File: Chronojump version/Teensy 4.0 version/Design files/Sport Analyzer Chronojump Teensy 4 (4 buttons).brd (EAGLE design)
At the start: 122.7 x 68.6 mm, 40 parts, among them IC2 7805DT, Q1 MMBT4403, Q2 BSS138, Q3 BSS138, SW1 C&K_COMPONENTS_D6R40F1LFSC&K_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, SW2 C&K_COMPONENTS_D6R40F1LFSC&K_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, SW3 C&K_COMPONENTS_D6R40F1LFSC&K_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, SW4 C&K_COMPONENTS_D6R40F1LFSC&K_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, U1 HX711

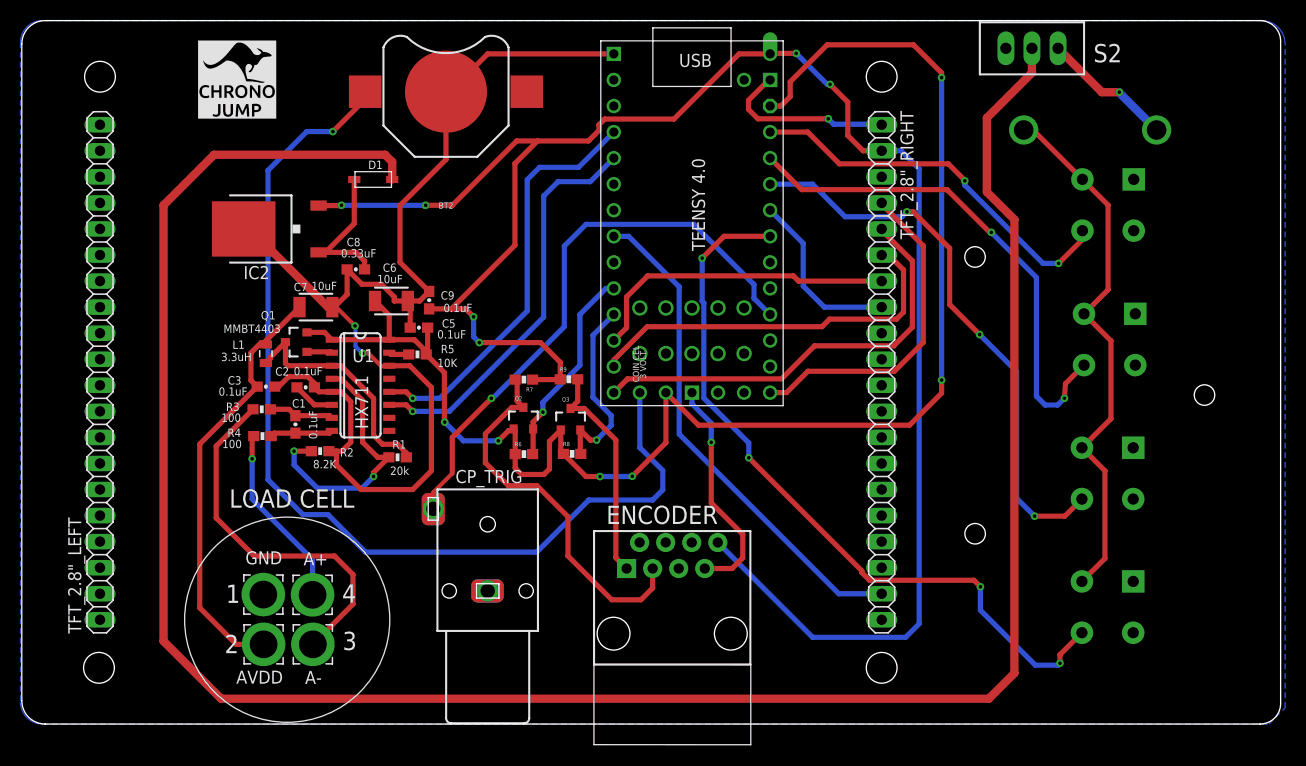
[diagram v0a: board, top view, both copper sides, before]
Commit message: RTC DS1302 v1
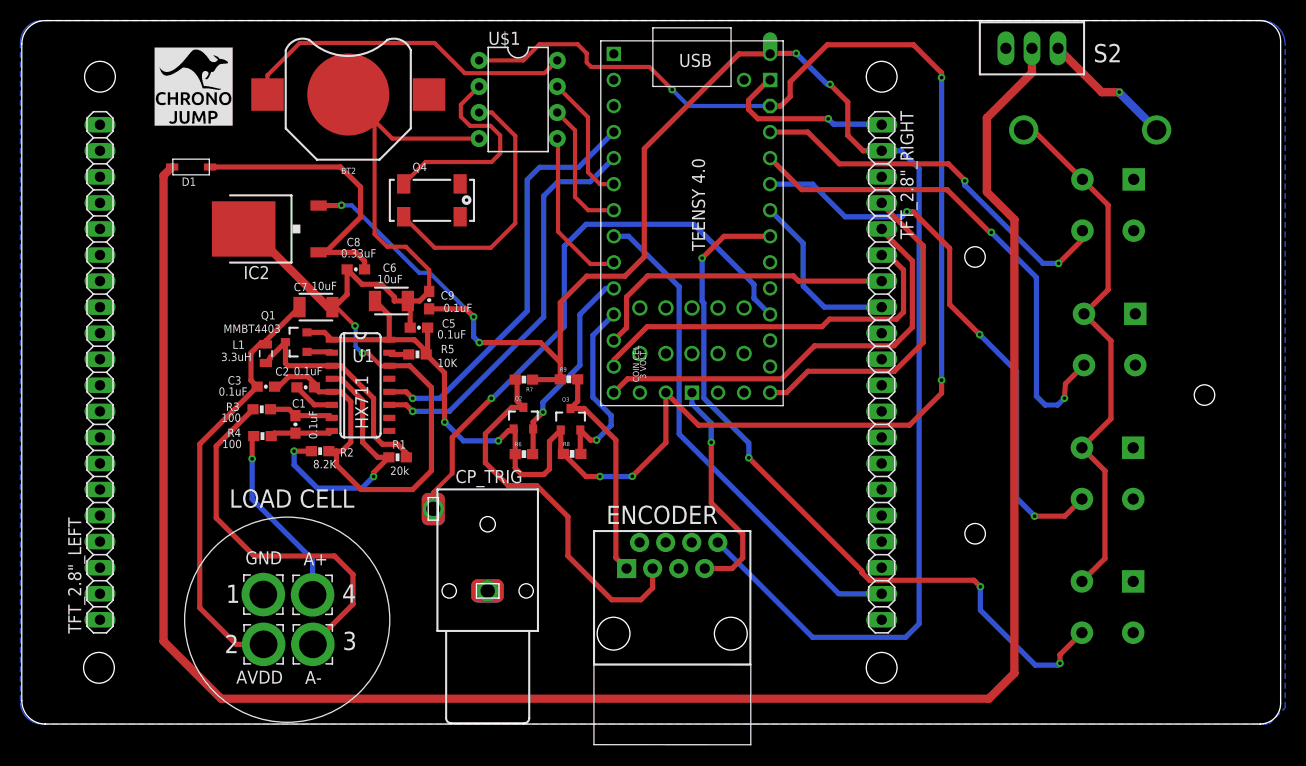
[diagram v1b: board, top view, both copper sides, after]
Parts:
- added Q4: 32.768, microbuilder:CRYSTAL_8X3.8
- added U$1: DS1302, adafruit:DIL08-ROUND
- moved D1 17.8 mm to (17.0, 55.1), turned to 180 degrees
- moved BT2 9.53 mm to (32.3, 62.1)
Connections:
- removed net N$14: BT2.PWR@1, U$2.VBAT
- new net N$18: BT2.PWR@1, U$1.8
- new net N$8: Q4.P$4, U$1.2
- new net N$9: Q4.P$1, U$1.3
- new net RTC_CE: U$1.5, U$2.7-RX2/OUT1A
- new net RTC_I/O: U$1.6, U$2.5-IN2
- new net RTC_SCLK: U$1.7, U$2.4-BCLK2
- net GND: now also U$1.4
- net VDD: now also U$1.1
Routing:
- net N$14: track 97.6 -> 0.00 mm, vias 1 -> 0
- net N$18: track 0.00 -> 33.2 mm
- net VDD: track 148.4 -> 180.5 mm, vias 6 -> 7
- net N$9: track 0.00 -> 26.1 mm
- net 9V: track 219.0 -> 196.7 mm
- net N$8: track 0.00 -> 20.7 mm
- net RTC_CE: track 0.00 -> 15.9 mm
- net 9VD: track 14.6 -> 29.6 mm
- net RTC_I/O: track 0.00 -> 13.3 mm
- net RTC_SCLK: track 0.00 -> 12.6 mm
- net VCC: track 180.4 -> 172.1 mm, vias 6 -> 5
- net GND: track 212.5 -> 206.4 mm
